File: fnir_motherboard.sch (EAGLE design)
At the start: 44 parts, among them IC1 LTC2494, IC3 AD712R, U2 ATMEGA8U2QFN, X2 USB-SMD-NS, Y1 16MHz

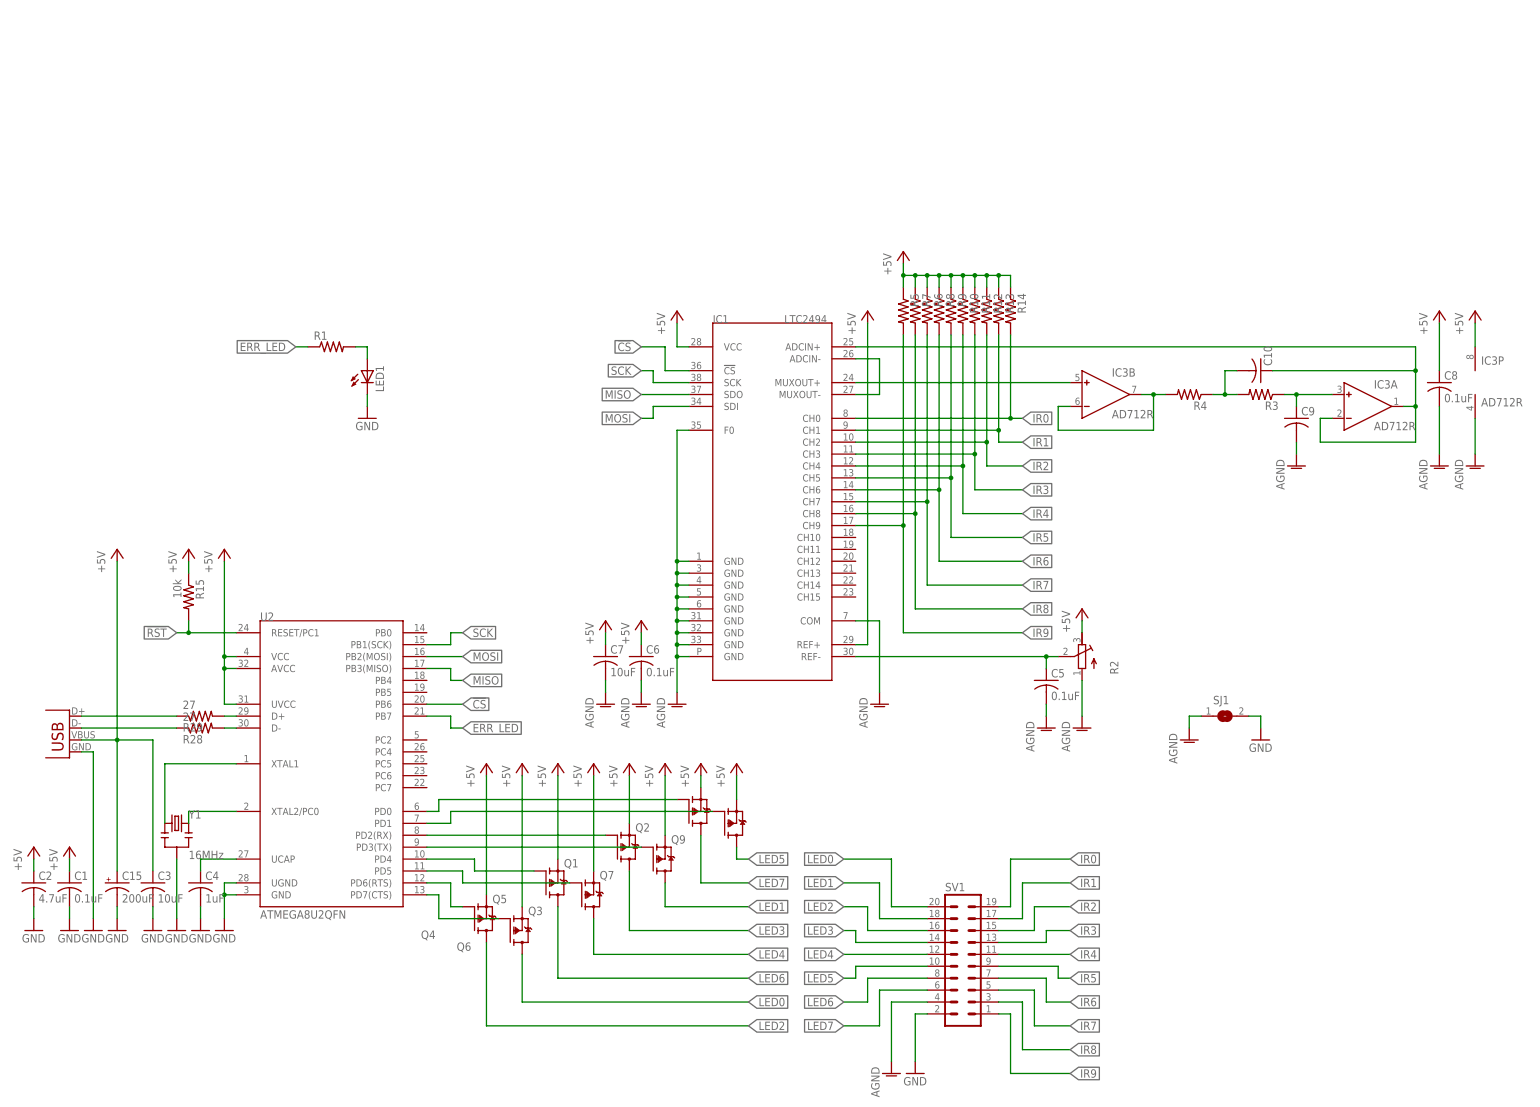
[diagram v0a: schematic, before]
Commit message: new version desinged
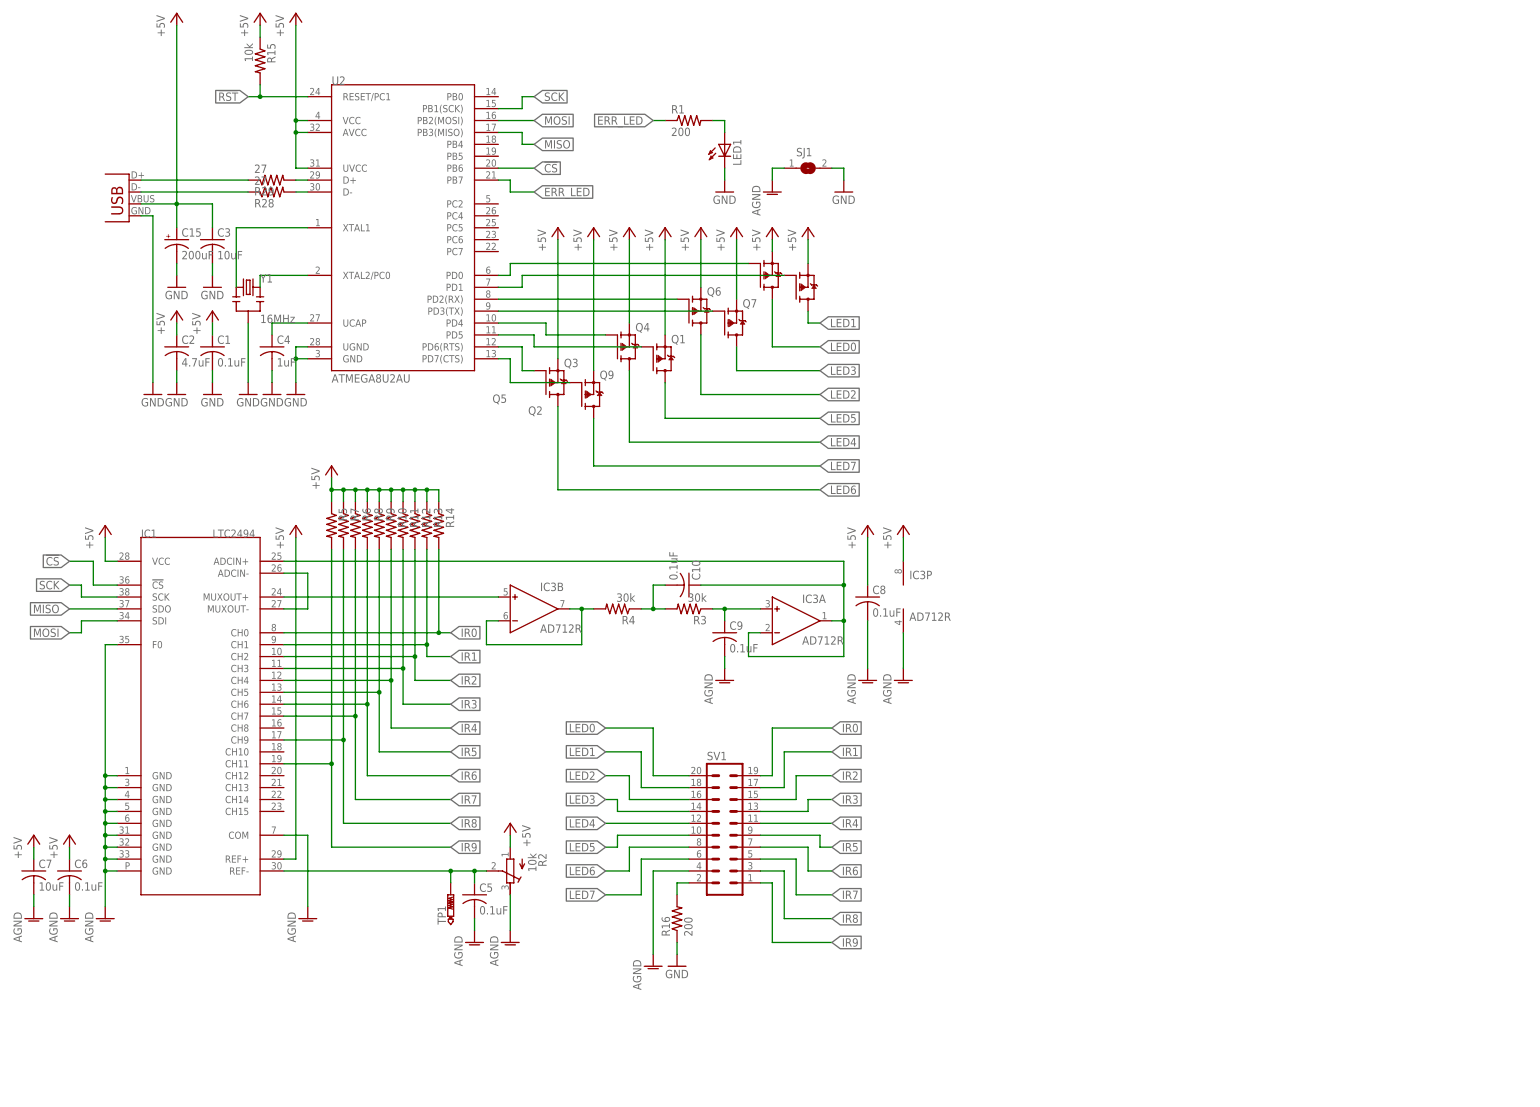
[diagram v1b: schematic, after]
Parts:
- added R16: 200, adafruit:R-US_R1206
- added TP1: PTR1B1,27, testpad:PTR1B1,27
- C1, C2, C3, C4, C5, C6, C7, C8: device adafruit:C-USC0805 -> adafruit:C-USC1206
- C10, C9: value (none) -> 0.1uF; device adafruit:C-USC0805 -> adafruit:C-USC1206
- R1: value (none) -> 200; device adafruit:R-US_R0805 -> adafruit:R-US_R1206
- R10, R11, R12, R13, R14, R15, R28, R29, R5, R6, R7, R8, R9: device adafruit:R-US_R0805 -> adafruit:R-US_R1206
- R2: value (none) -> 10k
- R3, R4: value (none) -> 30k; device adafruit:R-US_R0805 -> adafruit:R-US_R1206
- U2: value ATMEGA8U2QFN -> ATMEGA8U2AU; device sparkfun:ATMEGA8U2QFN -> sparkfun:ATMEGA8U2AU
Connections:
- new net N$23: R16.2, SV1.2
- net +5V: now also R2.A; no longer R2.E
- net AGND: now also R2.E; no longer R2.A
- net GND: now also R16.1; no longer SV1.2
- net IR8: now also IC1.CH9; no longer IC1.CH8
- net IR9: now also IC1.CH11; no longer IC1.CH9
- net N$1: now also Q2.G; no longer Q6.G
- net N$12: now also TP1.TP
- net N$2: now also Q1.G; no longer Q7.G
- net N$3: now also Q9.G, U2.PD5; no longer Q5.G, U2.PD4
- net N$4: now also Q4.G; no longer Q1.G
- net N$5: now also Q5.G; no longer Q4.G
- net N$6: now also Q7.G; no longer Q9.G
- net N$7: now also Q6.G; no longer Q2.G
- net N$8: now also U2.PD4; no longer U2.PD5
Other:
- moved on the sheet: C1, C10, C15, C2, C3, C4, C5, C6, C7, C8, C9, IC1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
